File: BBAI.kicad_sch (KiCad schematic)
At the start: 2 parts, among them P1 BBAI - P8, P2 BBAI - P9

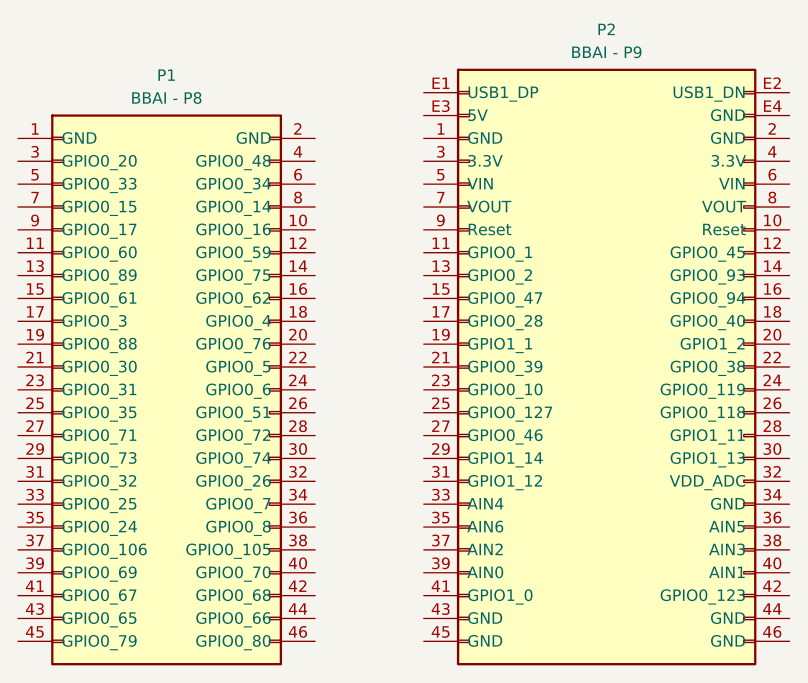
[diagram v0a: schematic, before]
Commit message: I don't know
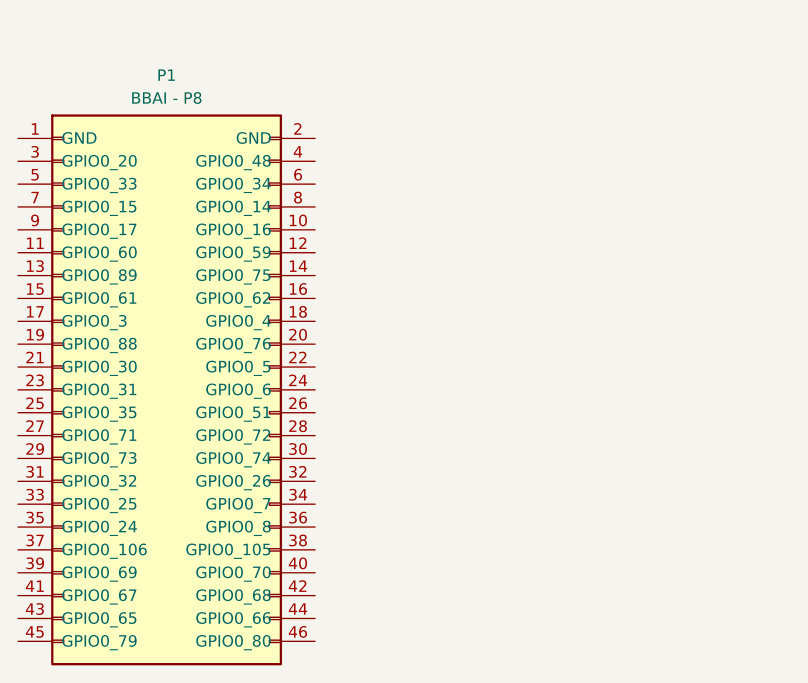
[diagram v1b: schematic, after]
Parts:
- removed P2: BBAI - P9, symbol Scout_library:BBAIP9
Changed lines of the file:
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@@
 (kicad_sch (version 20230121) (generator eeschema)
   (paper "A4")
-  (symbol (lib_name "BBAIP9_1") (lib_id "Scout_library:BBAIP9") (at 106.045 85.725 0) (unit 1)
-    (in_bom yes) (on_board yes) (dnp no) (fields_autoplaced)
-    (property "Reference" "P2" (at 121.285 48.26 0)
-      (effects (font (size 1.27 1.27)))
-    )
-    (property "Value" "BBAI - P9" (at 121.285 50.8 0)
-      (effects (font (size 1.27 1.27)))
-    )
-    (property "Footprint" "" (at 106.045 85.725 0)
-      (effects (font (size 1.27 1.27)) hide)
-    )
-    (property "Datasheet" "~" (at 106.045 85.725 0)
-      (effects (font (size 1.27 1.27)) hide)
-    )
-    (pin "2")
-    (pin "25")
-    (pin "27")
-    (pin "29")
-    (pin "36")
-    (pin "37")
-    (pin "28")
-    (pin "13")
-    (pin "17")
-    (pin "38")
-    (pin "39")
-    (pin "4")
-    (pin "11")
-    (pin "21")
-    (pin "40")
-    (pin "10")
-    (pin "41")
-    (pin "42")
-    (pin "43")
-    (pin "44")
-    (pin "35")
-    (pin "45")
-    (pin "46")
-    (pin "33")
-    (pin "5")
-    (pin "6")
-    (pin "3")
-    (pin "32")
-    (pin "20")
-    (pin "1")
-    (pin "18")
-    (pin "15")
-    (pin "23")
-    (pin "22")
-    (pin "16")
-    (pin "24")
-    (pin "26")
-    (pin "30")
-    (pin "31")
-    (pin "12")
-    (pin "19")
-    (pin "14")
-    (pin "34")
-    (pin "8")
-    (pin "9")
-    (pin "E2")
-    (pin "E4")
-    (pin "7")
-    (pin "E1")
-    (pin "E3")
-    (instances
-      (project "Scout_Board"
-        (path "/e58a9779-147f-4c0c-a745-6e9bc8ec0357/f69c0108-1493-406f-9c14-edf38ee5c388"
-          (reference "P2") (unit 1)
-        )
-      )
-    )
-  )
   (symbol (lib_name "BBAIP8_1") (lib_id "Scout_library:BBAIP8") (at 60.96 88.265 0) (unit 1)
     (in_bom yes) (on_board yes) (dnp no) (fields_autoplaced)
